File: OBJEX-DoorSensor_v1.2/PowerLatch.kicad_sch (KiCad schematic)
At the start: 23 parts, among them Q1 BC857B_RF, Q2 NTNUS3171PZT5G, Q3 2N7002KQBZ, U3 S-5701BC11B-L3T2U5, U4 SN74LVC1G86DBVR, U5 SN74LVC1G86DBVR

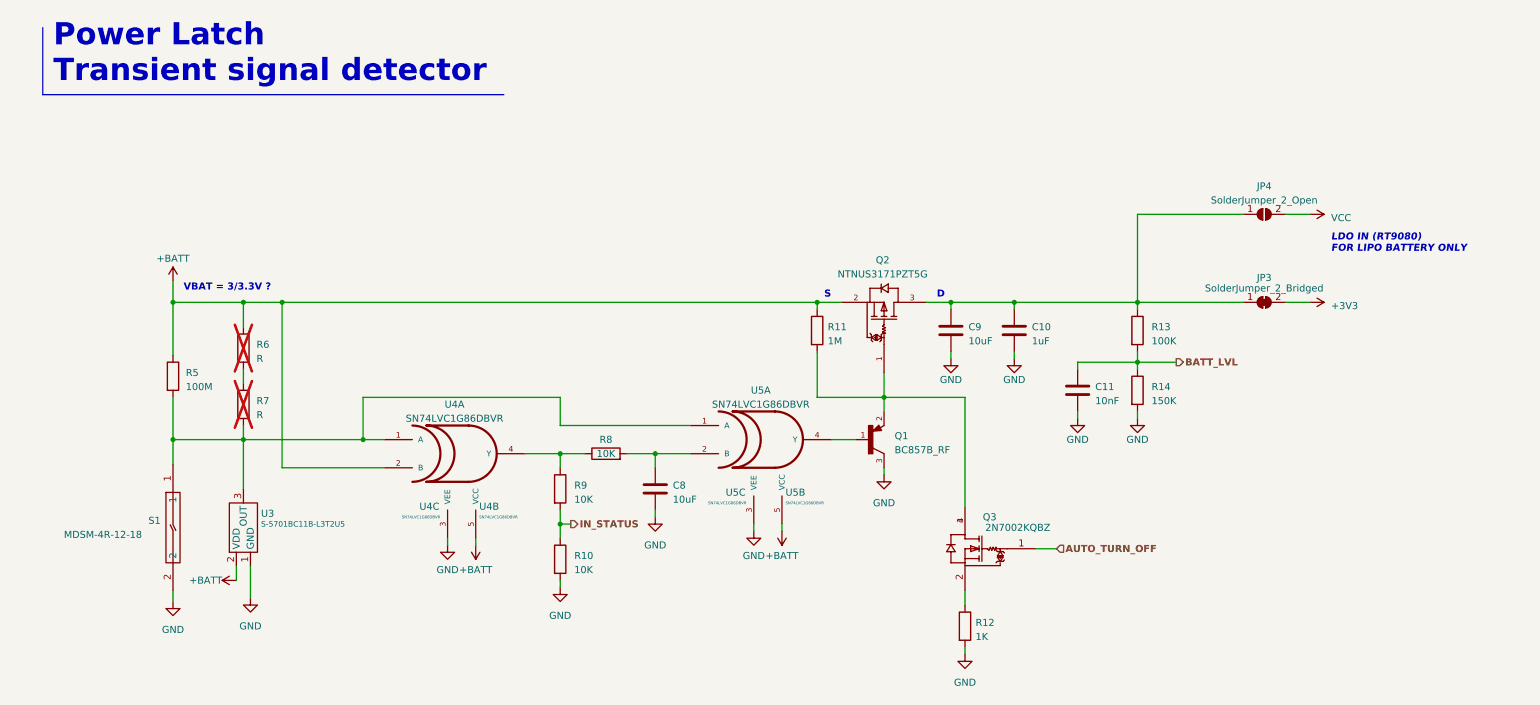
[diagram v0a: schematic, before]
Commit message: UPDATE
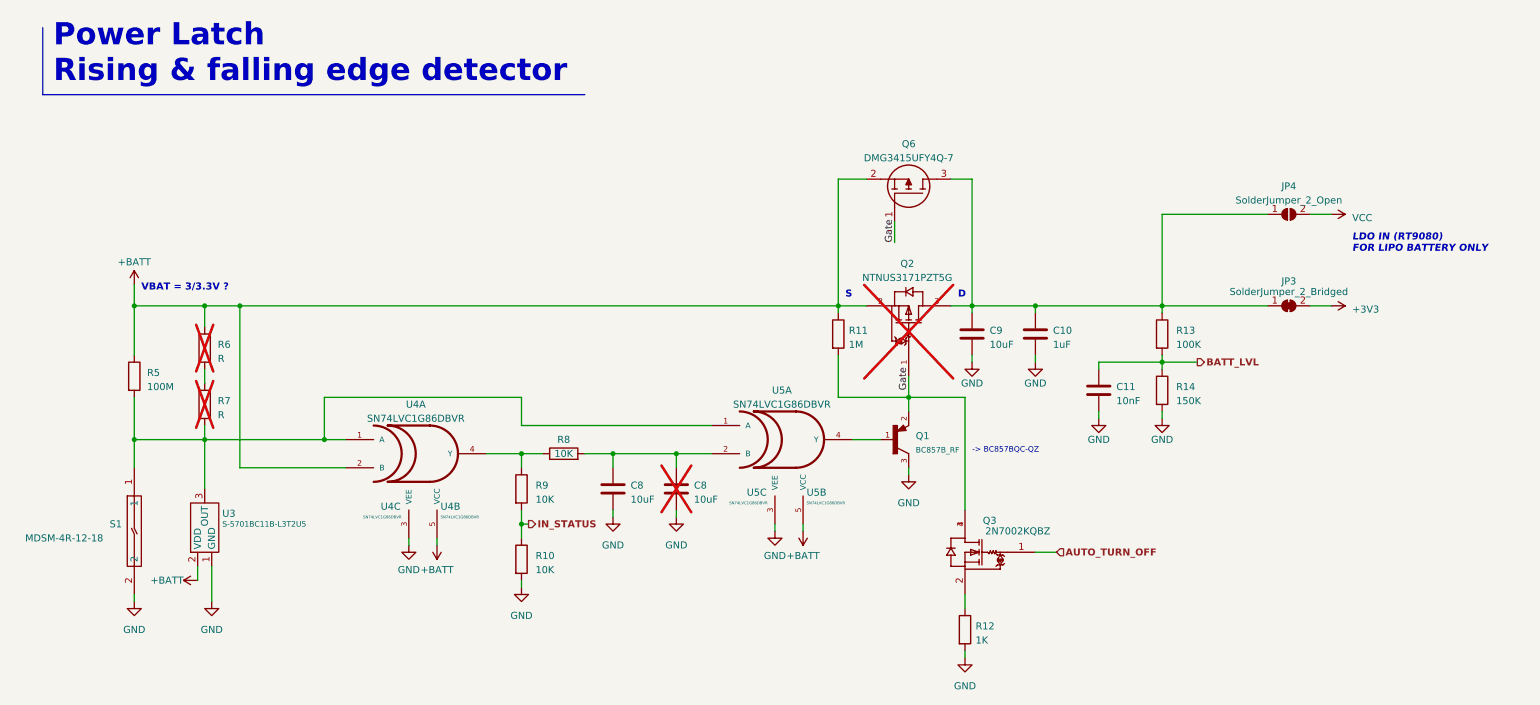
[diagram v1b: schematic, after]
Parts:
- added C8: 10uF, symbol Device:C
- added Q6: DMG3415UFY4Q-7, DMG3415UFY47, symbol DMG3415UFY4Q-7:DMG3415UFY4Q-7
- Q2: now not fitted
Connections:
- net +BATT: now also Q6.2
- net GND: now also C8.2
- net at C10.1, C9.1, JP3.1 (A)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: now also Q6.3
- net at C8.1, R8.2, U5.2 (B): now also C8.1
- net Gate: now reaches Q1.2, Q2.1, Q3.3, Q3.4, R11.2
- net Gate: now also Q6.1
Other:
- note added: "-> BC857BQC-QZ"
- note added: "Power Latch Rising & falling edge detector"
- note removed: "Power Latch Transient signal detector"
- moved on the sheet: C10, C11, C8, C9, JP3, JP4, Q1, Q3, R10, R11, R12, R13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

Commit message: Ready for components placing
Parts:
- C10, C8, C9: footprint (none) -> Capacitor_SMD:C_0603_1608Metric
- C11, C8: footprint (none) -> Capacitor_SMD:C_0402_1005Metric
- JP3: footprint (none) -> Jumper:SolderJumper-2_P1.3mm_Bridged_RoundedPad1.0x1.5mm
- JP4: footprint (none) -> Jumper:SolderJumper-2_P1.3mm_Open_RoundedPad1.0x1.5mm
- Q1: footprint SOT95P237X112-3N -> lib:SOT95P237X112-3N
- Q2: footprint ONSC-SOT-1123-3-524AA_V -> lib:ONSC-SOT-1123-3-524AA_V
- Q3: footprint 2N7002KQBZ -> lib:2N7002KQBZ
- Q6: footprint DMG3415UFY47 -> lib:DMG3415UFY47
- R10, R11, R12, R13, R14, R8, R9: footprint (none) -> Resistor_SMD:R_0402_1005Metric
- R5, R6, R7: footprint (none) -> Resistor_SMD:R_0603_1608Metric
- S1: footprint MDSM4R1218 -> lib:MDSM4R1218
- U3: footprint (none) -> Ablic:S'5701BC11B'L3T2U5
- U4, U5: footprint SOT353 -> lib:SOT353
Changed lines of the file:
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@@
       (effects (font (size 1.27 1.27)) (justify left))
     )
-    (property "Footprint" "" (at 219.202 85.09 90)
+    (property "Footprint" "Resistor_SMD:R_0402_1005Metric" (at 219.202 85.09 90)
       (effects (font (size 1.27 1.27)) hide)
     )
@@
       (effects (font (size 1.27 1.27)) (justify left))
     )
-    (property "Footprint" "" (at 199.0852 78.74 0)
+    (property "Footprint" "Capacitor_SMD:C_0603_1608Metric" (at 199.0852 78.74 0)
       (effects (font (size 1.27 1.27)) hide)
     )
@@
       (effects (font (size 0.5 0.5)) (justify right))
     )
-    (property "Footprint" "SOT353" (at 85.09 106.68 0)
+    (property "Footprint" "lib:SOT353" (at 85.09 106.68 0)
       (effects (font (size 1.27 1.27)) (justify bottom) hide)
     )
@@
       (effects (font (size 1.27 1.27)) (justify left))
     )
-    (property "Footprint" "" (at 210.5152 88.9 0)
+    (property "Footprint" "Capacitor_SMD:C_0402_1005Metric" (at 210.5152 88.9 0)
       (effects (font (size 1.27 1.27)) hide)
     )
@@
       (effects (font (size 1.27 1.27)) (justify left))
     )
-    (property "Footprint" "" (at 33.782 82.55 90)
+    (property "Footprint" "Resistor_SMD:R_0603_1608Metric" (at 33.782 82.55 90)
       (effects (font (size 1.27 1.27)) hide)
     )
@@
       (effects (font (size 1.27 1.27)) (justify left))
     )
-    (property "Footprint" "" (at 122.8852 106.68 0)
+    (property "Footprint" "Capacitor_SMD:C_0603_1608Metric" (at 122.8852 106.68 0)
       (effects (font (size 1.27 1.27)) hide)
     )
@@
       (effects (font (size 0.5 0.5)) (justify right))
     )
-    (property "Footprint" "SOT353" (at 156.21 104.14 0)
+    (property "Footprint" "lib:SOT353" (at 156.21 104.14 0)
       (effects (font (size 1.27 1.27)) (justify bottom) hide)
     )
@@
       (effects (font (size 1.27 1.27)))
     )
-    (property "Footprint" "" (at 243.84 69.85 0)
+    (property "Footprint" "Jumper:SolderJumper-2_P1.3mm_Bridged_RoundedPad1.0x1.5mm" (at 243.84 69.85 0)
       (effects (font (size 1.27 1.27)) hide)
     )
@@
       (effects (font (size 1.27 1.27)))
     )
-    (property "Footprint" "SOT353" (at 78.74 101.6 0)
+    (property "Footprint" "lib:SOT353" (at 78.74 101.6 0)
       (effects (font (size 1.27 1.27)) (justify bottom) hide)
     )
@@
       (effects (font (size 1.27 1.27)))
     )
-    (property "Footprint" "" (at 243.84 53.34 0)
+    (property "Footprint" "Jumper:SolderJumper-2_P1.3mm_Open_RoundedPad1.0x1.5mm" (at 243.84 53.34 0)
       (effects (font (size 1.27 1.27)) hide)
     )
@@
       (effects (font (size 1.27 1.27)) (justify left))
     )
-    (property "Footprint" "" (at 160.782 74.93 90)
+    (property "Footprint" "Resistor_SMD:R_0402_1005Metric" (at 160.782 74.93 90)
       (effects (font (size 1.27 1.27)) hide)
     )
@@
       (effects (font (size 1.27 1.27)))
     )
-    (property "Footprint" "ONSC-SOT-1123-3-524AA_V" (at 177.8 77.47 0)
+    (property "Footprint" "lib:ONSC-SOT-1123-3-524AA_V" (at 177.8 77.47 0)
       (effects (font (size 1.27 1.27)) (justify bottom) hide)
     )
@@
       (effects (font (size 1.27 1.27)) (justify left))
     )
-    (property "Footprint" "" (at 46.482 87.63 90)
+    (property "Footprint" "Resistor_SMD:R_0603_1608Metric" (at 46.482 87.63 90)
       (effects (font (size 1.27 1.27)) hide)
     )
@@
       (effects (font (size 1.27 1.27)))
     )
-    (property "Footprint" "SOT353" (at 144.78 99.06 0)
+    (property "Footprint" "lib:SOT353" (at 144.78 99.06 0)
       (effects (font (size 1.27 1.27)) (justify bottom) hide)
     )
@@
       (effects (font (size 1.27 1.27)) (justify left))
     )
-    (property "Footprint" "" (at 134.3152 106.68 0)
+    (property "Footprint" "Capacitor_SMD:C_0402_1005Metric" (at 134.3152 106.68 0)
       (effects (font (size 1.27 1.27)) hide)
     )
@@
       (effects (font (size 1.27 1.27)))
     )
-    (property "Footprint" "2N7002KQBZ" (at 166.37 110.49 0)
+    (property "Footprint" "lib:2N7002KQBZ" (at 166.37 110.49 0)
       (effects (font (size 1.27 1.27)) (justify left) hide)
     )
@@
       (effects (font (size 1.27 1.27)) (justify left))
     )
-    (property "Footprint" "" (at 103.632 115.57 90)
+    (property "Footprint" "Resistor_SMD:R_0402_1005Metric" (at 103.632 115.57 90)
       (effects (font (size 1.27 1.27)) hide)
     )
@@
       (effects (font (size 1.27 1.27)) (justify left))
     )
-    (property "Footprint" "" (at 103.632 102.87 90)
+    (property "Footprint" "Resistor_SMD:R_0402_1005Metric" (at 103.632 102.87 90)
       (effects (font (size 1.27 1.27)) hide)
     )
@@
       (effects (font (size 1.27 1.27)) (justify left))
     )
-    (property "Footprint" "" (at 187.6552 78.74 0)
+    (property "Footprint" "Capacitor_SMD:C_0603_1608Metric" (at 187.6552 78.74 0)
       (effects (font (size 1.27 1.27)) hide)
     )
@@
       (effects (font (size 0.5 0.5)) (justify right))
     )
-    (property "Footprint" "SOT353" (at 151.13 104.14 0)
+    (property "Footprint" "lib:SOT353" (at 151.13 104.14 0)
       (effects (font (size 1.27 1.27)) (justify bottom) hide)
     )
@@
       (effects (font (size 1.27 1.27)))
     )
-    (property "Footprint" "" (at 113.03 98.298 90)
+    (property "Footprint" "Resistor_SMD:R_0402_1005Metric" (at 113.03 98.298 90)
       (effects (font (size 1.27 1.27)) hide)
     )
@@
       (effects (font (size 1.27 1.27)) (justify left))
     )
-    (property "Footprint" "" (at 183.642 128.27 90)
+    (property "Footprint" "Resistor_SMD:R_0402_1005Metric" (at 183.642 128.27 90)
       (effects (font (size 1.27 1.27)) hide)
     )
@@
       (effects (font (size 0.5 0.5)) (justify right))
     )
-    (property "Footprint" "SOT353" (at 90.17 106.68 0)
+    (property "Footprint" "lib:SOT353" (at 90.17 106.68 0)
       (effects (font (size 1.27 1.27)) (justify bottom) hide)
     )
@@
       (effects (font (size 1.27 1.27)) (justify left))
     )
-    (property "Footprint" "" (at 219.202 74.93 90)
+    (property "Footprint" "Resistor_SMD:R_0402_1005Metric" (at 219.202 74.93 90)
       (effects (font (size 1.27 1.27)) hide)
     )
@@
       (effects (font (size 1.27 1.27)) (justify left))
     )
-    (property "Footprint" "MDSM4R1218" (at 52.07 106.68 0)
+    (property "Footprint" "lib:MDSM4R1218" (at 52.07 106.68 0)
       (effects (font (size 1.27 1.27)) (justify left) hide)
     )
@@
       (effects (font (size 1.27 1.27)))
     )
-    (property "Footprint" "DMG3415UFY47" (at 171.45 43.18 0)
+    (property "Footprint" "lib:DMG3415UFY47" (at 171.45 43.18 0)
       (effects (font (size 1.27 1.27)) (justify left) hide)
     )
@@
       (effects (font (size 1.27 1.27)) (justify left))
     )
-    (property "Footprint" "" (at 46.482 77.47 90)
+    (property "Footprint" "Resistor_SMD:R_0603_1608Metric" (at 46.482 77.47 90)
       (effects (font (size 1.27 1.27)) hide)
     )
@@
       (effects (font (size 1 1)) (justify left))
     )
-    (property "Footprint" "SOT95P237X112-3N" (at 172.72 93.98 0)
+    (property "Footprint" "lib:SOT95P237X112-3N" (at 172.72 93.98 0)
       (effects (font (size 1.27 1.27)) (justify bottom) hide)
     )
@@
       (effects (font (size 1 1)) (justify right))
     )
-    (property "Footprint" "" (at 43.18 109.22 0)
-      (effects (font (size 1.27 1.27)) hide)
-    )
+    (property "Footprint" "Ablic:S'5701BC11B'L3T2U5" (at 43.18 109.22 0)
+      (effects (font (size 1.27 1.27)) hide)
+    )

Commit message: update
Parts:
- C10, C9: footprint Capacitor_SMD:C_0603_1608Metric -> Capacitor_SMD:C_0402_1005Metric
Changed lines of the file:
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@@
       (effects (font (size 1.27 1.27)) (justify left))
     )
-    (property "Footprint" "Capacitor_SMD:C_0603_1608Metric" (at 199.0852 78.74 0)
+    (property "Footprint" "Capacitor_SMD:C_0402_1005Metric" (at 199.0852 78.74 0)
       (effects (font (size 1.27 1.27)) hide)
     )
@@
       (effects (font (size 1.27 1.27)) (justify left))
     )
-    (property "Footprint" "Capacitor_SMD:C_0603_1608Metric" (at 187.6552 78.74 0)
-      (effects (font (size 1.27 1.27)) hide)
-    )
+    (property "Footprint" "Capacitor_SMD:C_0402_1005Metric" (at 187.6552 78.74 0)
+      (effects (font (size 1.27 1.27)) hide)
+    )

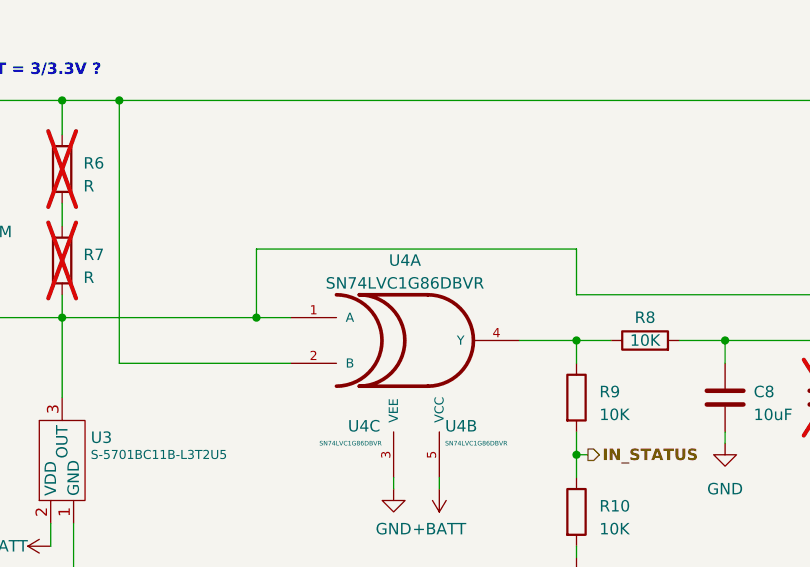
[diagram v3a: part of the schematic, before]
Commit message: Ready for order
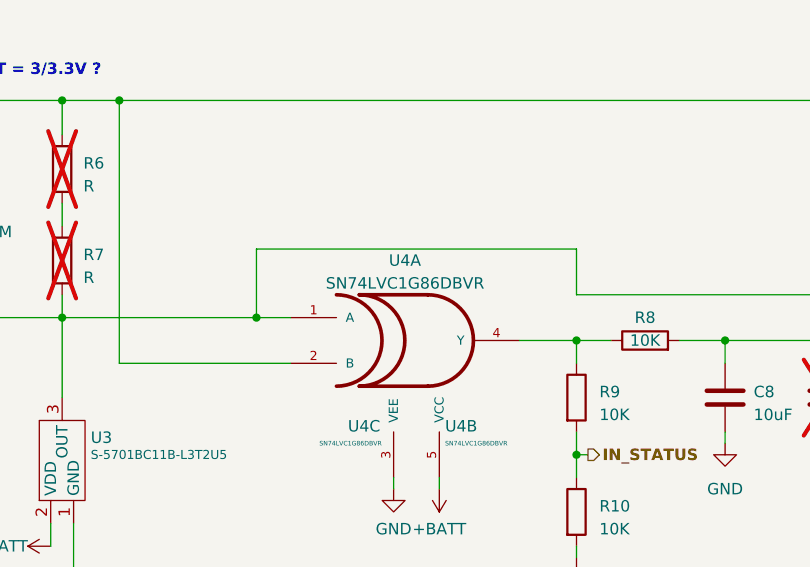
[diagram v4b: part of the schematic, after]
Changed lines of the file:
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@@
   )
   (symbol (lib_id "SN74LVC1G86DBVR:SN74LVC1G86DBVR") (at 78.74 101.6 0) (unit 1)
-    (in_bom yes) (on_board yes) (dnp no) (fields_autoplaced)
+    (in_bom yes) (on_board yes) (dnp no)
     (property "Reference" "U4" (at 86.3489 87.63 0)
       (effects (font (size 1.27 1.27)))
     )
-    (property "Value" "SN74LVC1G86DBVR" (at 86.3489 90.17 0)
+    (property "Value" "SN74LVC1G86DBVR" (at 86.36 90.17 0)
       (effects (font (size 1.27 1.27)))
     )

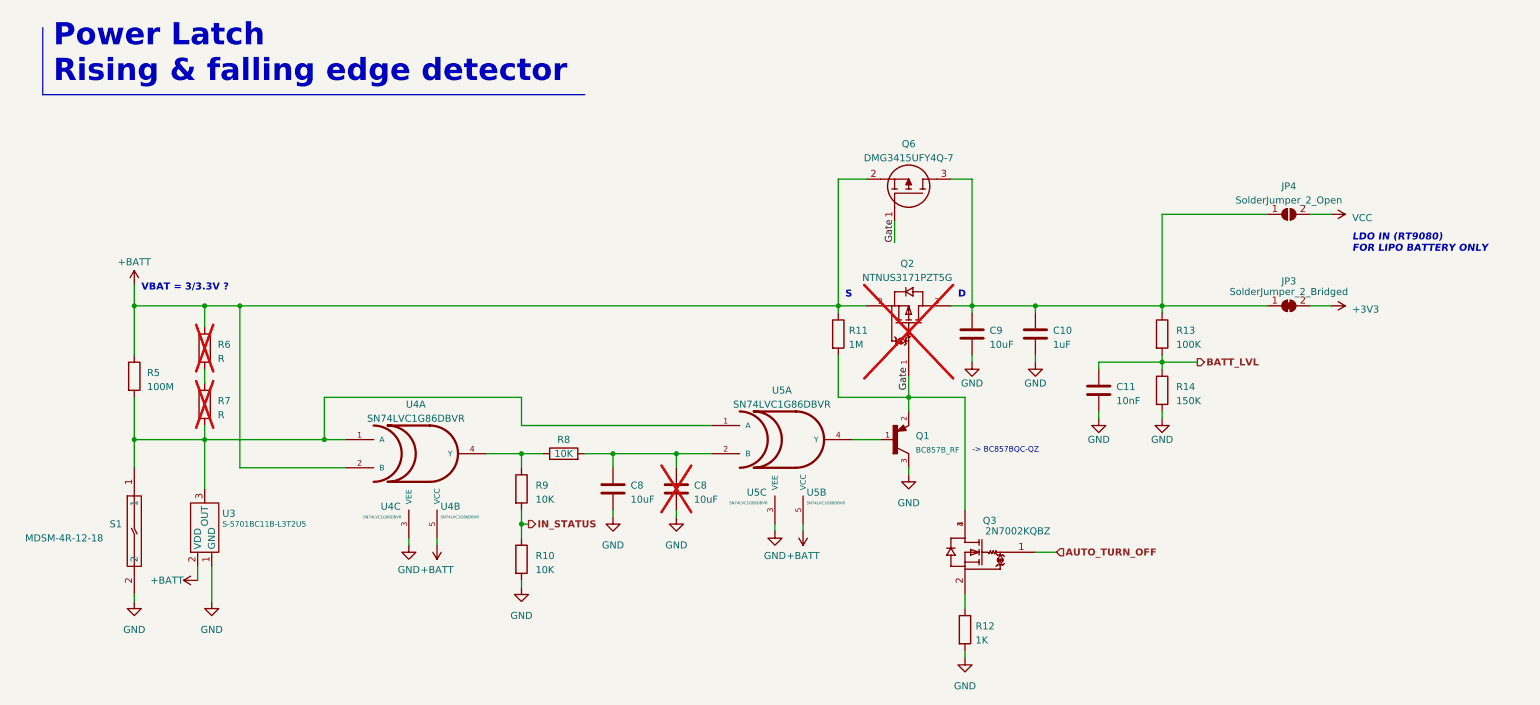
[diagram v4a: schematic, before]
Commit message: Final review - ready for production
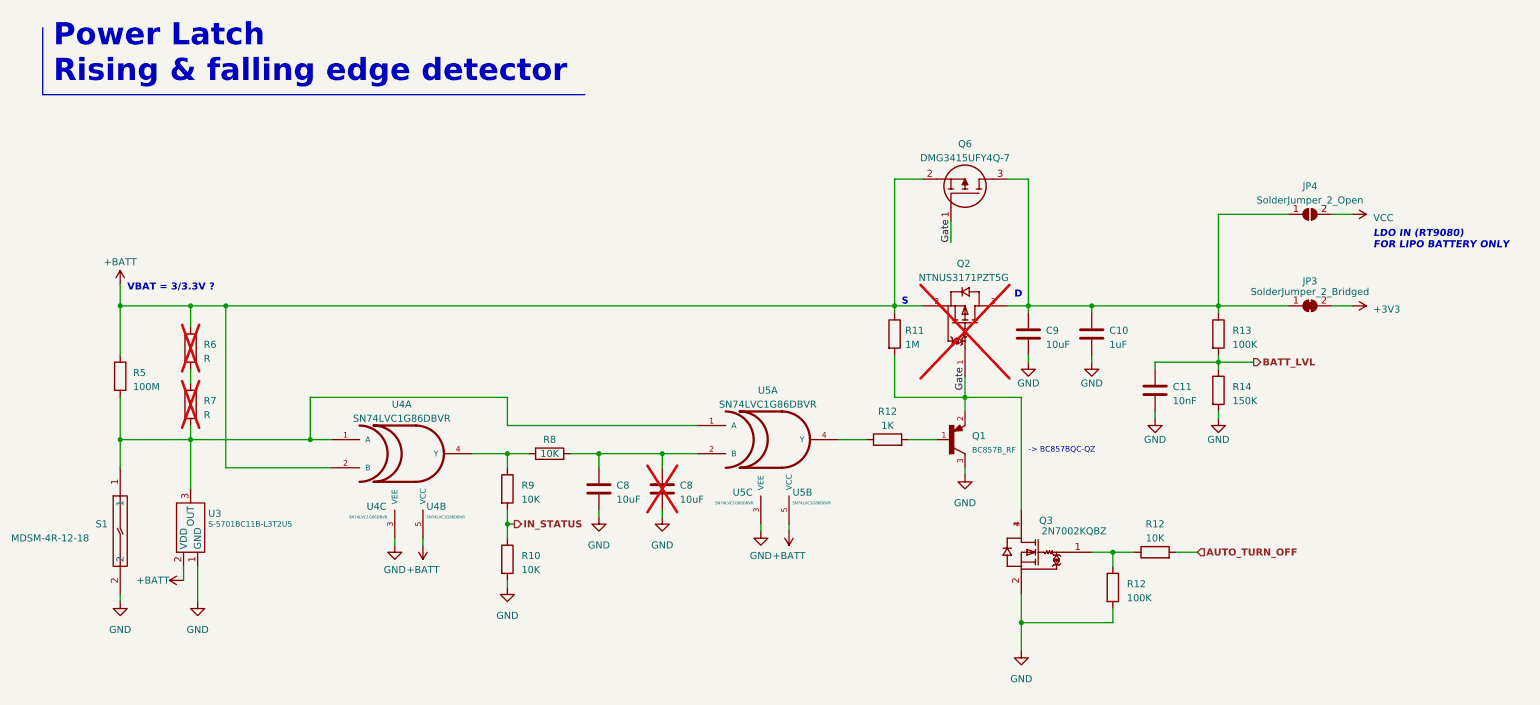
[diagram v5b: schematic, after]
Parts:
- removed R12: 1K, Resistor_SMD:R_0402_1005Metric, symbol Device:R
- added R12: 100K, Resistor_SMD:R_0402_1005Metric, symbol Device:R
- added R12: 1K, Resistor_SMD:R_0402_1005Metric, symbol Device:R
- added R12: 10K, Resistor_SMD:R_0402_1005Metric, symbol Device:R
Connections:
- net AUTO_TURN_OFF: now also R12.2; no longer Q3.1
- net GND: now also Q3.2, R12.2
- net at U5.4 (Y): now also R12.1; no longer Q1.1
- new net: Q3.1, R12.1, R12.1
- new net: Q1.1, R12.2
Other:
- moved on the sheet: C10, C11, C8, C9, JP3, JP4, Q1, Q2, Q3, Q6, R10, R11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
